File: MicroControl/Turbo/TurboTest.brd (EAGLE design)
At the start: 13.9 x 10.1 mm, 9 parts, among them IC1 555

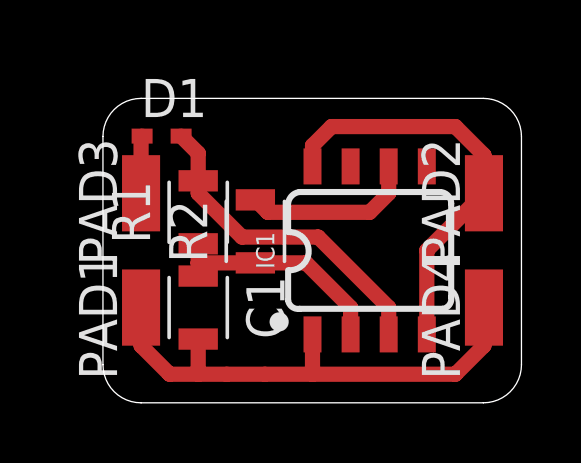
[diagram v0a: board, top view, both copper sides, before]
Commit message: 3D
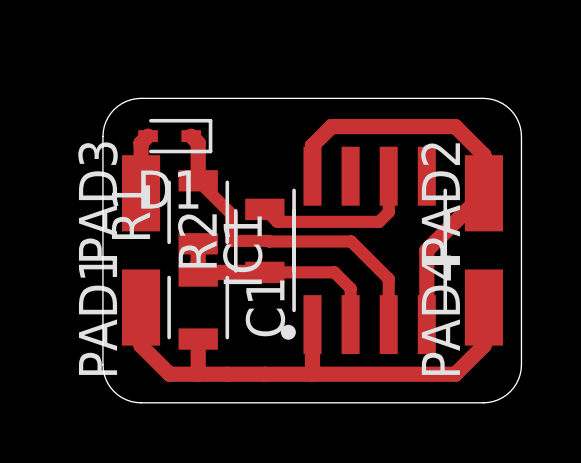
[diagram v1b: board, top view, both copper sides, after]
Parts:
- D1: device Flamberm:SOD523 -> Flamberm:SODFL1608X65
- IC1: device SparkFun-IC-Special-Function:SO08 -> Flamberm:SOIC-8
- moved R2 0.45 mm to (5.40, 5.40)
- moved D1 0.32 mm to (2.22, 8.89), turned to 180 degrees
- turned IC1 to 90 degrees
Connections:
- net N$3: now also D1.1; no longer D1.A
- net N$4: now also D1.2; no longer D1.C
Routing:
- net N$3: track 11.0 -> 11.9 mm
- net N$1: track 7.67 -> 8.47 mm
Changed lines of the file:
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@@
 </layers>
 <board>
-<fusionsync huburn="a.cGVyc29uYWw6dWUyOGRlMGUz" projecturn="a.cGVyc29uYWw6dWUyOGRlMGUzIzIwMTcwNDA2NzA3MTU3MDY" f3durn="urn:adsk.wipprod:dm.lineage:fojqi3iZSGGzgwdvYKWH5w" pcbguid="132616ee-cdcb-4346-af84-ddefcf6b20db" lastpulledtime="" lastsyncedchangeguid="e96ec202-4e3c-405b-30bf-2fbe633682c4"/>
+<fusionsync huburn="a.cGVyc29uYWw6dWUyOGRlMGUz" projecturn="a.cGVyc29uYWw6dWUyOGRlMGUzIzIwMTcwNDA2NzA3MTU3MDY" f3durn="urn:adsk.wipprod:dm.lineage:fojqi3iZSGGzgwdvYKWH5w" pcbguid="132616ee-cdcb-4346-af84-ddefcf6b20db" lastpulledtime="" lastsyncedchangeguid="2cf39450-8c5b-74ef-8fd0-1515978d6d25"/>
 <plain>
 <wire x1="0" y1="8.8775" x2="0" y2="1.27" width="0" layer="20"/>
@@
 <elements>
 <element name="C1" library="Flamberm" library_urn="urn:adsk.eagle:library:2654185" package="CAP0805" package3d_urn="urn:adsk.eagle:package:4015421/2" value="1u" x="3.175" y="3.175" rot="R270"/>
-<element name="D1" library="Flamberm" library_urn="urn:adsk.eagle:library:2654185" package="SOD523" package3d_urn="urn:adsk.eagle:package:2654517/1" value="" x="1.905" y="8.89"/>
-<element name="IC1" library="SparkFun-IC-Special-Function" library_urn="urn:adsk.eagle:library:527" package="SO08" package3d_urn="urn:adsk.eagle:package:39192/1" value="555" x="8.89" y="5.08">
-<attribute name="PROD_ID" value="NA-XXXXX" x="8.89" y="5.08" size="1.778" layer="27" display="off"/>
-</element>
+<element name="D1" library="Flamberm" library_urn="urn:adsk.eagle:library:2654185" package="SODFL1608X65" package3d_urn="urn:adsk.eagle:package:4109696/1" value="" x="2.2225" y="8.89" rot="R180"/>
+<element name="IC1" library="Flamberm" library_urn="urn:adsk.eagle:library:2654185" package="SOIC-8" package3d_urn="urn:adsk.eagle:package:4108622/2" value="555" x="8.89" y="5.08" rot="R90"/>
 <element name="PAD1" library="wirepad" library_urn="urn:adsk.eagle:library:412" package="SMD1,27-2,54" package3d_urn="urn:adsk.eagle:package:30839/1" value="WIREPADSMD1,27-254" x="1.27" y="3.175"/>
 <element name="PAD2" library="wirepad" library_urn="urn:adsk.eagle:library:412" package="SMD1,27-2,54" package3d_urn="urn:adsk.eagle:package:30839/1" value="WIREPADSMD1,27-254" x="12.7" y="6.985"/>
@@
 <element name="PAD4" library="wirepad" library_urn="urn:adsk.eagle:library:412" package="SMD1,27-2,54" package3d_urn="urn:adsk.eagle:package:30839/1" value="WIREPADSMD1,27-254" x="12.7" y="3.175"/>
 <element name="R1" library="Flamberm" library_urn="urn:adsk.eagle:library:2654185" package="RESC2012X50" package3d_urn="urn:adsk.eagle:package:4015756/1" value="50K" x="3.175" y="6.35" rot="R90"/>
-<element name="R2" library="Flamberm" library_urn="urn:adsk.eagle:library:2654185" package="RESC2012X50" package3d_urn="urn:adsk.eagle:package:4015756/1" value="0" x="5.08" y="5.715" rot="R90"/>
+<element name="R2" library="Flamberm" library_urn="urn:adsk.eagle:library:2654185" package="RESC2012X50" package3d_urn="urn:adsk.eagle:package:4015756/1" value="0" x="5.3975" y="5.3975" rot="R90"/>
 </elements>
 <signals>
@@
 <wire x1="12.7" y1="8.255" x2="11.7475" y2="9.2075" width="0.508" layer="1"/>
 <wire x1="12.7" y1="6.985" x2="10.795" y2="5.08" width="0.508" layer="1"/>
-<wire x1="10.795" y1="5.08" x2="10.795" y2="2.28" width="0.508" layer="1"/>
+<wire x1="10.795" y1="5.08" x2="10.795" y2="2.6066" width="0.508" layer="1"/>
 <wire x1="11.7475" y1="9.2075" x2="7.62" y2="9.2075" width="0.508" layer="1"/>
 <wire x1="7.62" y1="9.2075" x2="6.985" y2="8.5725" width="0.508" layer="1"/>
-<wire x1="6.985" y1="8.5725" x2="6.985" y2="7.88" width="0.508" layer="1"/>
+<wire x1="6.985" y1="8.5725" x2="6.985" y2="7.5534" width="0.508" layer="1"/>
 </signal>
 <signal name="N$1">
@@
 <wire x1="3.175" y1="4.445" x2="3.175" y2="4.225" width="0.508" layer="1"/>
 <contactref element="R2" pad="1"/>
-<wire x1="5.08" y1="4.665" x2="3.175" y2="4.665" width="0.508" layer="1"/>
-<wire x1="5.08" y1="4.665" x2="6.765" y2="4.665" width="0.508" layer="1"/>
-<wire x1="6.765" y1="4.665" x2="8.255" y2="3.175" width="0.508" layer="1"/>
-<wire x1="8.255" y1="3.175" x2="8.255" y2="2.28" width="0.508" layer="1"/>
+<wire x1="5.3975" y1="4.3475" x2="3.175" y2="4.3475" width="0.508" layer="1"/>
+<wire x1="8.255" y1="3.175" x2="8.255" y2="2.6066" width="0.508" layer="1"/>
 <wire x1="3.175" y1="4.665" x2="3.175" y2="4.445" width="0.508" layer="1"/>
+<wire x1="3.175" y1="4.665" x2="3.175" y2="4.3475" width="0.508" layer="1"/>
+<wire x1="5.3975" y1="4.3475" x2="7.7175" y2="4.3475" width="0.4064" layer="1"/>
+<wire x1="7.7175" y1="4.3475" x2="8.255" y2="3.81" width="0.4064" layer="1"/>
+<wire x1="8.255" y1="3.81" x2="8.255" y2="2.6066" width="0.4064" layer="1"/>
 </signal>
 <signal name="GND">
@@
 <wire x1="1.27" y1="1.905" x2="1.27" y2="3.175" width="0.508" layer="1"/>
 <wire x1="3.175" y1="2.125" x2="3.175" y2="0.9525" width="0.508" layer="1"/>
-<wire x1="6.985" y1="2.28" x2="6.985" y2="0.9525" width="0.508" layer="1"/>
+<wire x1="6.985" y1="2.6066" x2="6.985" y2="0.9525" width="0.508" layer="1"/>
 <wire x1="6.985" y1="0.9525" x2="5.3975" y2="0.9525" width="0.508" layer="1"/>
 <wire x1="3.175" y1="0.9525" x2="2.2225" y2="0.9525" width="0.508" layer="1"/>
@@
 <contactref element="IC1" pad="3"/>
 <contactref element="R1" pad="2"/>
-<contactref element="D1" pad="A"/>
-<wire x1="2.605" y1="8.89" x2="3.175" y2="8.32" width="0.508" layer="1"/>
-<wire x1="3.175" y1="8.32" x2="3.175" y2="7.4" width="0.508" layer="1"/>
-<wire x1="3.175" y1="7.4" x2="3.175" y2="6.985" width="0.508" layer="1"/>
-<wire x1="4.6351" y1="5.5249" x2="7.1751" y2="5.5249" width="0.508" layer="1"/>
-<wire x1="7.1751" y1="5.5249" x2="9.525" y2="3.175" width="0.508" layer="1"/>
-<wire x1="9.525" y1="3.175" x2="9.525" y2="2.28" width="0.508" layer="1"/>
-<wire x1="3.175" y1="6.985" x2="4.6351" y2="5.5249" width="0.508" layer="1"/>
+<contactref element="D1" pad="1"/>
+<wire x1="9.525" y1="3.175" x2="9.525" y2="2.6066" width="0.508" layer="1"/>
+<wire x1="2.9426" y1="8.89" x2="3.175" y2="8.6576" width="0.508" layer="1"/>
+<wire x1="3.175" y1="8.6576" x2="3.175" y2="7.4" width="0.508" layer="1"/>
+<wire x1="3.175" y1="7.4" x2="4.2841" y2="6.2909" width="0.4064" layer="1"/>
+<wire x1="4.2841" y1="6.2909" x2="4.2841" y2="5.3975" width="0.4064" layer="1"/>
+<wire x1="4.2841" y1="5.3975" x2="5.51920625" y2="5.3975" width="0.4064" layer="1"/>
+<wire x1="5.51920625" y1="5.3975" x2="5.54060625" y2="5.3761" width="0.4064" layer="1"/>
+<wire x1="5.54060625" y1="5.3761" x2="8.2764" y2="5.3761" width="0.4064" layer="1"/>
+<wire x1="8.2764" y1="5.3761" x2="9.525" y2="4.1275" width="0.4064" layer="1"/>
+<wire x1="9.525" y1="4.1275" x2="9.525" y2="2.6066" width="0.4064" layer="1"/>
 </signal>
 <signal name="N$4">
-<contactref element="D1" pad="C"/>
+<contactref element="D1" pad="2"/>
 <contactref element="PAD3" pad="1"/>
-<wire x1="1.27" y1="6.985" x2="1.27" y2="8.855" width="0.508" layer="1"/>
-<wire x1="1.27" y1="8.855" x2="1.305" y2="8.89" width="0.508" layer="1"/>
+<wire x1="1.5024" y1="8.89" x2="1.27" y2="8.6576" width="0.508" layer="1"/>
+<wire x1="1.27" y1="8.6576" x2="1.27" y2="6.985" width="0.508" layer="1"/>
 </signal>
 <signal name="N$2">
 <contactref element="IC1" pad="6"/>
 <contactref element="R2" pad="2"/>
-<wire x1="9.525" y1="7.88" x2="9.525" y2="6.985" width="0.508" layer="1"/>
-<wire x1="9.525" y1="6.985" x2="8.89" y2="6.35" width="0.508" layer="1"/>
-<wire x1="8.89" y1="6.35" x2="5.495" y2="6.35" width="0.508" layer="1"/>
-<wire x1="5.495" y1="6.35" x2="5.08" y2="6.765" width="0.508" layer="1"/>
+<wire x1="9.525" y1="6.985" x2="9.525" y2="7.5534" width="0.508" layer="1"/>
+<wire x1="5.3975" y1="6.4475" x2="5.8125" y2="6.0325" width="0.4064" layer="1"/>
+<wire x1="9.2075" y1="6.0325" x2="9.525" y2="6.35" width="0.4064" layer="1"/>
+<wire x1="9.525" y1="6.35" x2="9.525" y2="7.5534" width="0.4064" layer="1"/>
+<wire x1="5.8125" y1="6.0325" x2="9.2075" y2="6.0325" width="0.4064" layer="1"/>
 </signal>
 </signals>
